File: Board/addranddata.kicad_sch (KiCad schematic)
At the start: 64 parts, among them SW10 SW_SPDT, SW11 SW_SPDT, SW12 SW_SPDT, SW13 SW_SPDT, SW14 SW_SPDT, SW15 SW_SPDT, SW16 SW_SPDT, SW17 SW_SPDT, SW2 SW_SPDT, SW3 SW_SPDT, SW4 SW_SPDT, SW5 SW_SPDT, SW6 SW_SPDT, SW7 SW_SPDT, SW8 SW_SPDT, SW9 SW_SPDT

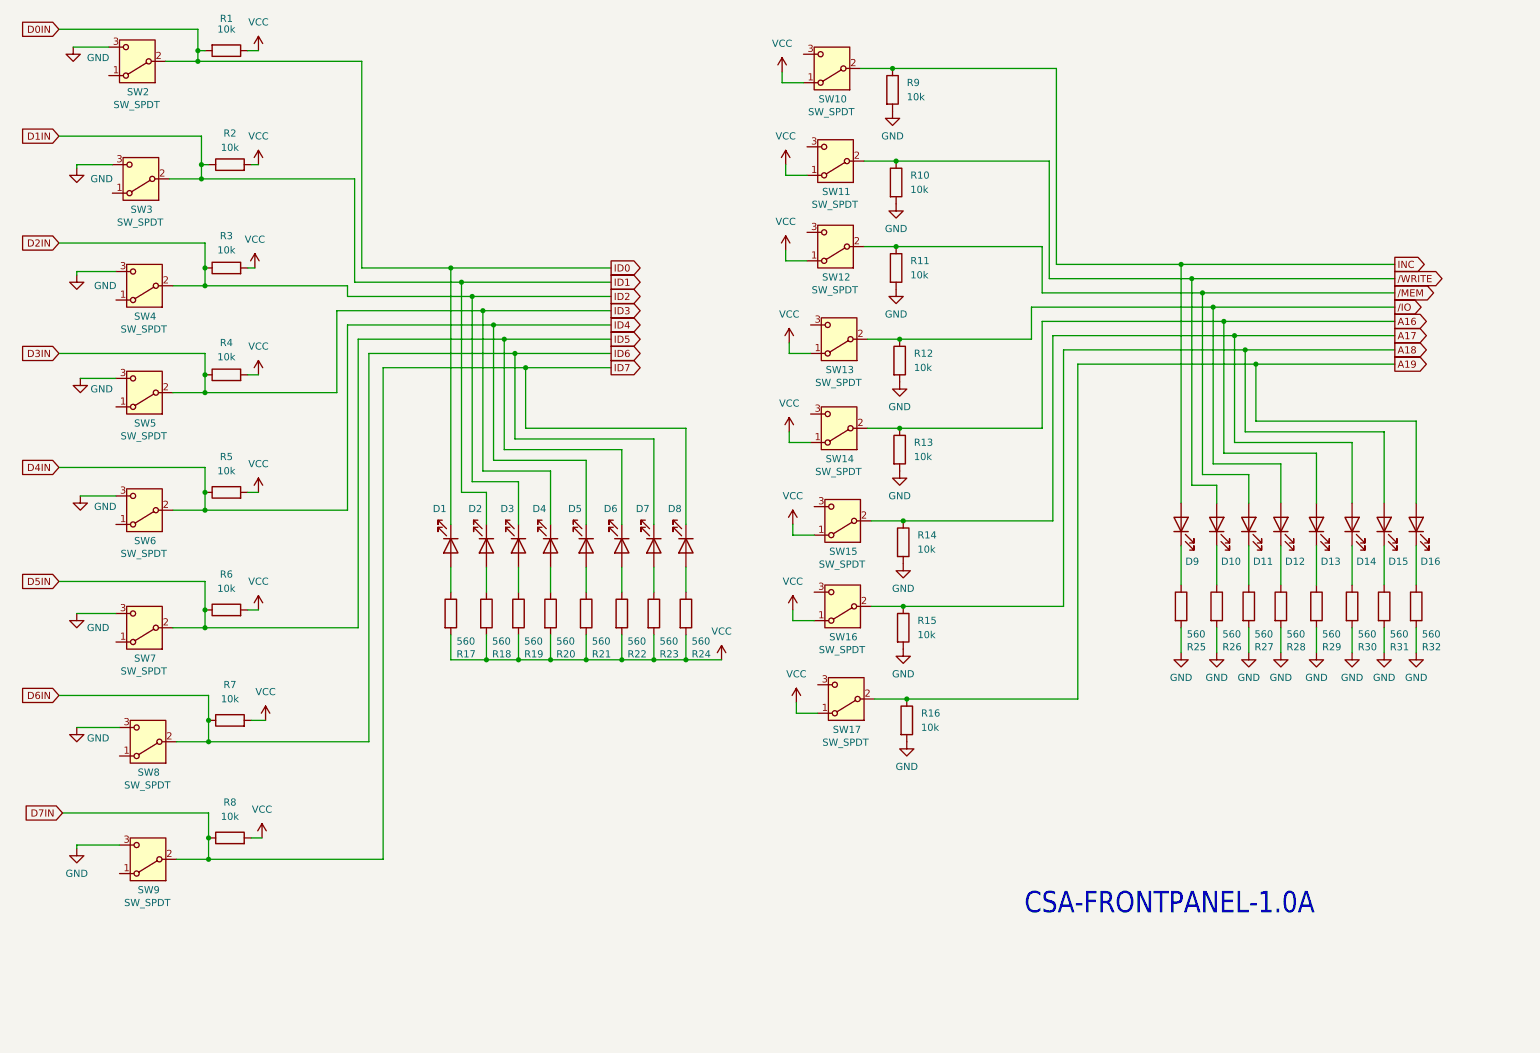
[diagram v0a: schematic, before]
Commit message: More work
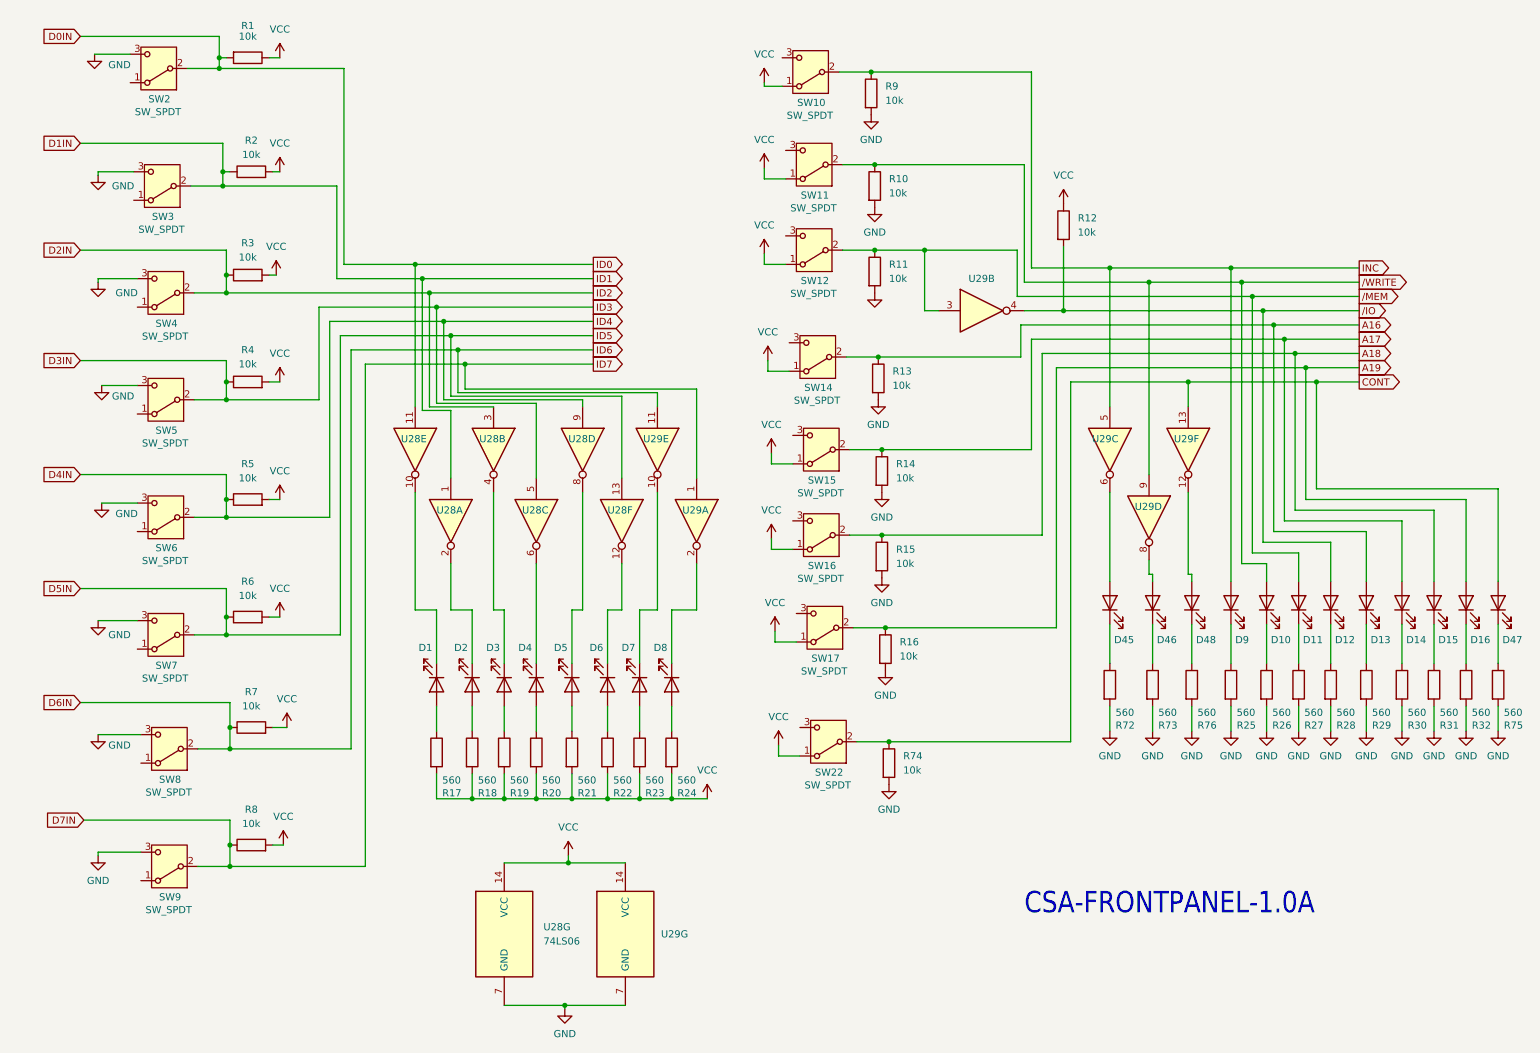
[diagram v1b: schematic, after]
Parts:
- removed SW13: SW_SPDT, Library:SW_K4625, symbol Switch:SW_SPDT
- added D45, D46, D47, D48: LED, LED_SMD:LED_0805_2012Metric_Pad1.15x1.40mm_HandSolder, symbol Device:LED
- added R72, R73, R75, R76: 560, Resistor_SMD:R_0603_1608Metric_Pad0.98x0.95mm_HandSolder, symbol Device:R
- added R74: 10k, Resistor_SMD:R_0603_1608Metric_Pad0.98x0.95mm_HandSolder, symbol Device:R
- added SW22: SW_SPDT, Library:SW_K4625, symbol Switch:SW_SPDT
- added U28, U29: 74LS06, Package_SO:SOIC-14_3.9x8.7mm_P1.27mm, symbol 74xx:74LS06
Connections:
- net D0IN: now also U28.11; no longer D1.1 (K)
- net D1IN: now also U28.1; no longer D2.1 (K)
- net D2IN: now also U28.3; no longer D3.1 (K)
- net D3IN: now also U28.5; no longer D4.1 (K)
- net D4IN: now also U28.9; no longer D5.1 (K)
- net D5IN: now also U28.13; no longer D6.1 (K)
- net D6IN: now also U29.11; no longer D7.1 (K)
- net D7IN: now also U29.1; no longer D8.1 (K)
- net GND: now also R72.2, R73.2, R74.2, R75.2, R76.2, U28.7 (GND), U29.7 (GND); no longer R12.2
- net INC: now also U29.5
- net VCC: now also R12.1, SW22.1 (A), U28.14 (VCC), U29.14 (VCC)
- net /IO: now also R12.2, U29.4; no longer R12.1
- net /MEM: now also U29.3
- net /WRITE: now also U29.9
- new net: D47.1 (K), R75.1
- new net: D5.1 (K), U28.8
- new net: D8.1 (K), U29.2
- new net: D3.1 (K), U28.4
- new net: D45.1 (K), R72.1
- new net: D45.2 (A), U29.6
- new net: D6.1 (K), U28.12
- new net: D46.1 (K), R73.1
- new net: D46.2 (A), U29.8
- new net: D48.1 (K), R76.1
- new net: D48.2 (A), U29.12
- new net: D1.1 (K), U28.10
- new net: D7.1 (K), U29.10
- new net: D2.1 (K), U28.2
- new net: D4.1 (K), U28.6
- new net CONT: D47.2 (A), R74.1, SW22.2 (B), U29.13
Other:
- moved on the sheet: D1, D10, D11, D12, D13, D14, D15, D16, D2, D3, D4, D5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
